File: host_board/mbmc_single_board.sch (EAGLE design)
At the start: 117 parts, among them IC1 ULN2803, IC15 PIC18F57K42-E_PT, IC16 REF3440IDBVR, IC17 MAX232, IC2 DIP Socket, IC3 REF02 5 VOLTS, IC4 5 VOLTS, IC5 12 VOLTS, IC6 3.3 VOLTS, J1 1-1586043-4, J2 1586044-4, Q3 ASF1, X15 RX-2, X16 TX-2, X17 RESETJMP, X20 PORTB

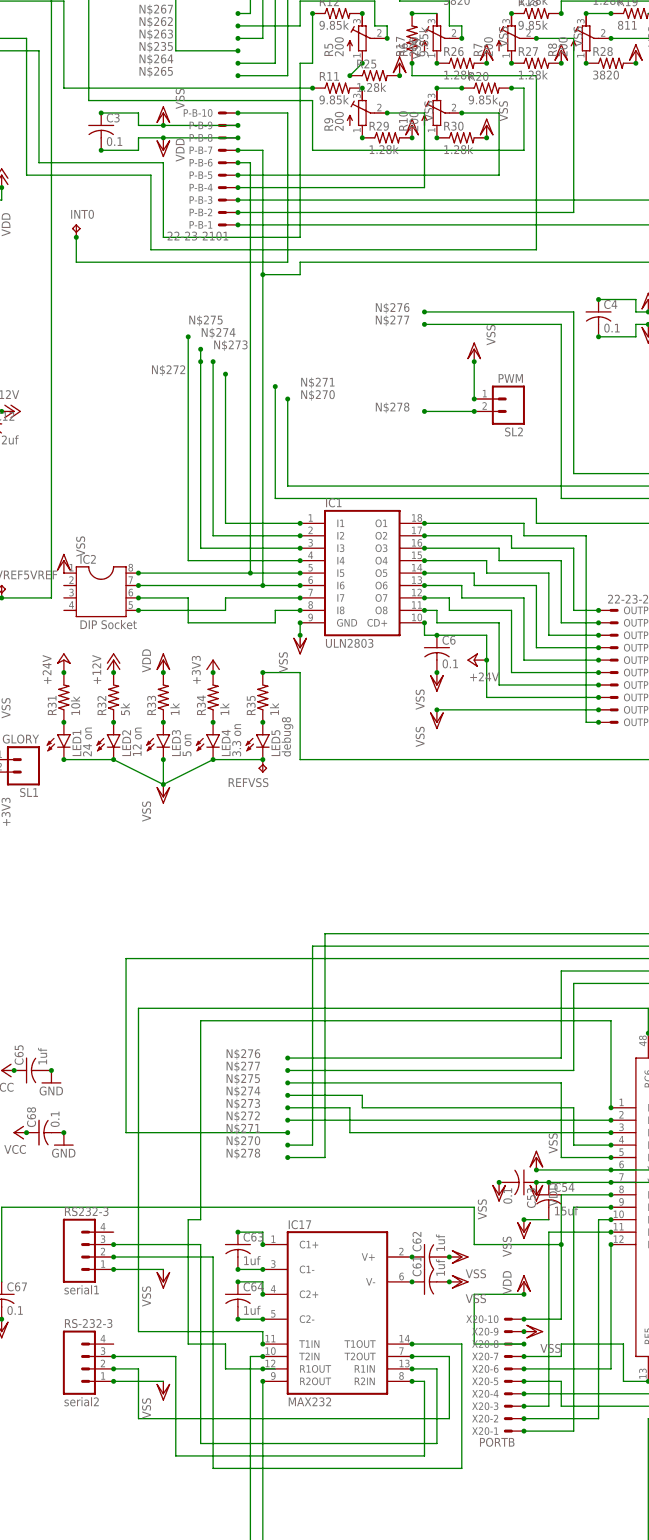
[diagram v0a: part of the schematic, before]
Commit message: up
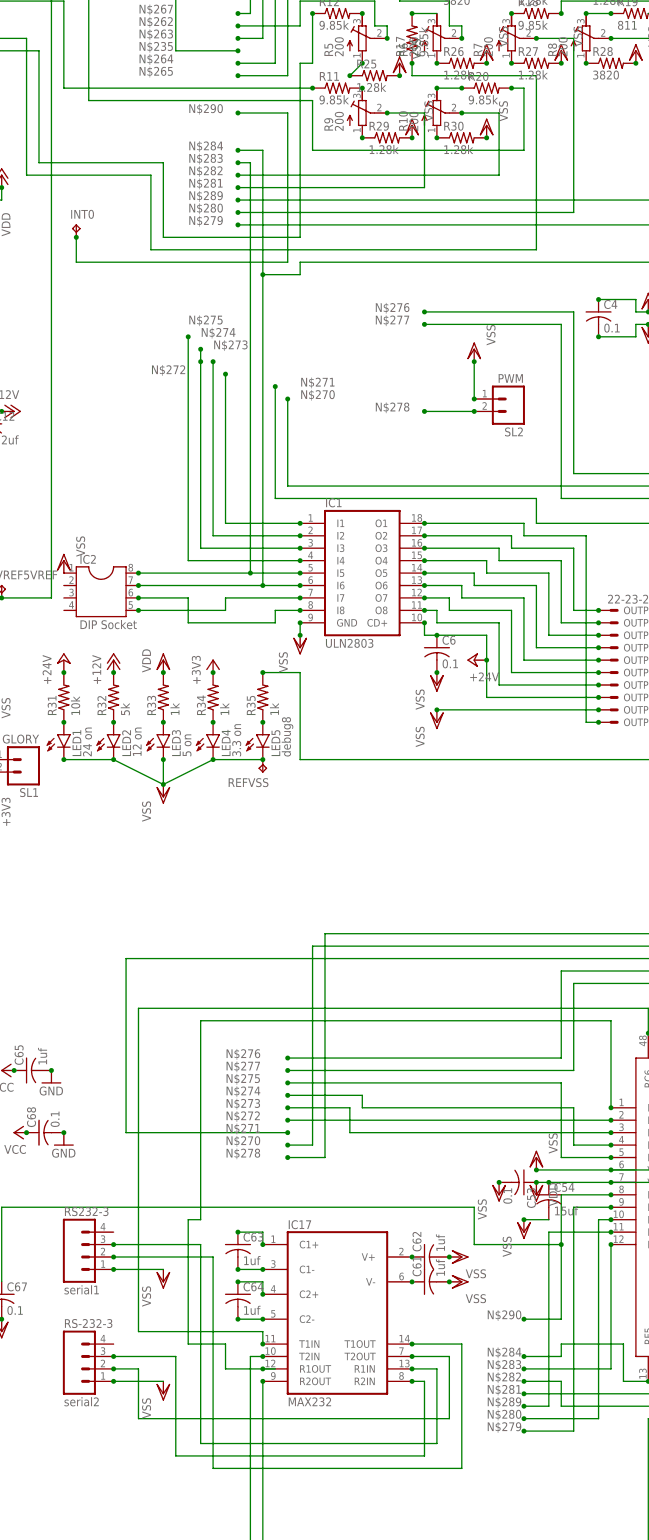
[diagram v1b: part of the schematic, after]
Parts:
- removed C3: 0.1, rcl:C-USC0805
- removed P-B: 22-23-2101, con-molex:22-23-2101
- removed X20: PORTB, con-molex:22-23-2101
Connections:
- removed net N$27: P-B-2.S, R7.S
- removed net N$28: P-B-3.S, R8.S
- removed net N$29: P-B-4.S, R9.S
- removed net N$30: P-B-5.S, R10.S
- removed net N$35: IC1.I5, IC2.8, P-B-6.S
- removed net N$36: IC1.I6, IC2.7, P-B-7.S, U$1.EN_L
- removed net N$40: P-B-1.S, U$1.CH_L
- removed net N$87: INT0.TP, P-B-10.S
- net N$279: now also U$1.CH_L; no longer X20-1.S
- net N$280: now also R7.S; no longer X20-2.S
- net N$281: now also R9.S; no longer X20-4.S
- net N$282: now also R10.S; no longer X20-5.S
- net N$283: now also IC1.I5, IC2.8; no longer X20-6.S
- net N$284: now also IC1.I6, IC2.7, U$1.EN_L; no longer X20-7.S
- net N$289: now also R8.S; no longer X20-3.S
- net N$290: now also INT0.TP; no longer X20-10.S
- net VDD: no longer C3.2, P-B-8.S, X20-8.S
- net VSS: no longer C3.1, P-B-9.S, X20-9.S
